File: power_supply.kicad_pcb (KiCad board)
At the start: 2 copper layers, 101.6 x 76.2 mm, 96 parts, among them J1 USB IN, J2 USB OUT, Q1 SI4174DY, Q2 SI4463CDY, Q3 SI4463CDY, U1 LM3914, U10 FDC6392S, U11 MCP6041, U2 TPD2E001, U3 MIC2185, U4 MCP73833, U5 TPD2E001, U6 TPS2511, U7 BATT, U8 LT1389, U9 MAX9938

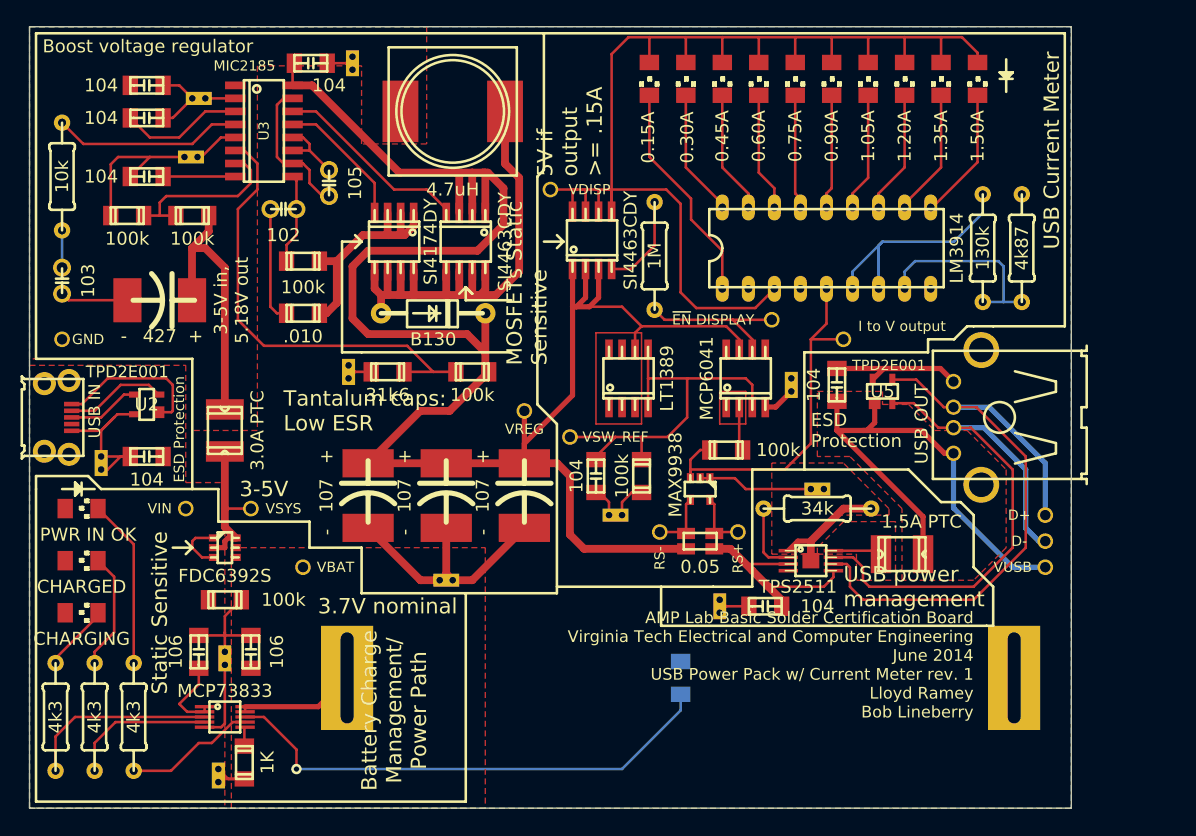
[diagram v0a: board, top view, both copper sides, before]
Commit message: Reshaping board
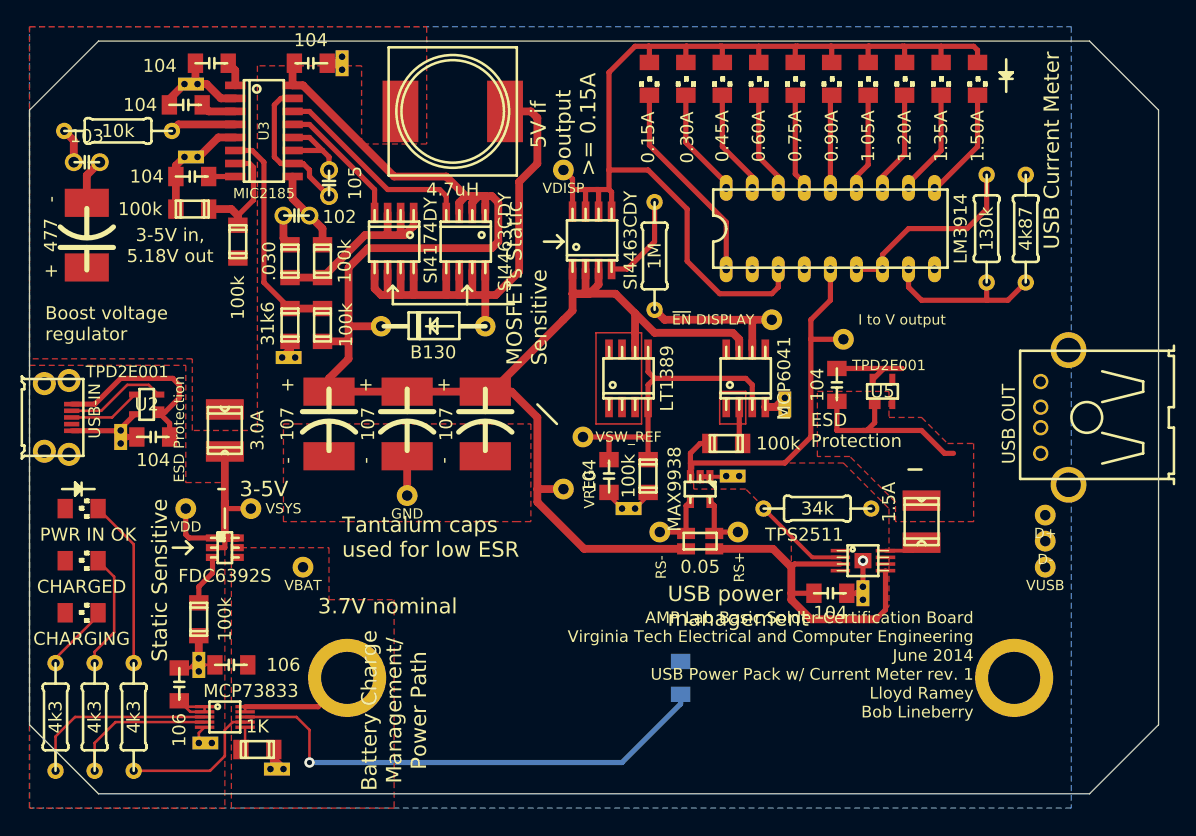
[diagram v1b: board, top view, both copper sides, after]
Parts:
- C1: value 427 -> 477
- D11: value CHARGED -> CHARGED
- F1: value 3.0A PTC -> 3.0A
- F2: value 1.5A PTC -> 1.5A
- J1: value USB IN -> USB-IN
- R10: value .010 -> .030
- RT1: value 10K -> 10K THERMISTOR
- TP1: value VIN -> VDD
- V12: value DV -> DBL_VIA
- moved TP14 36.9 mm to (189.2, 147.3)
- moved V5 28.4 mm to (169.5, 171.4)
- moved R13 15.3 mm to (181.0, 130.7), turned to 270 degrees
- moved V11 14.0 mm to (233.7, 156.8)
- moved C4 11.8 mm to (158.0, 114.8), turned to 0 degrees
- moved R14 10.6 mm to (177.8, 130.7), turned to 90 degrees
- moved C1 9.53 mm to (158.0, 121.9), turned to 90 degrees
- moved TP5 8.52 mm to (204.5, 146.7), turned to 180 degrees
- moved J2 8.51 mm to (262.5, 139.7)
- moved V10 8.35 mm to (221.0, 145.4)
- moved C12 7.96 mm to (196.8, 140.3)
- moved C14 7.96 mm to (189.2, 140.3)
- moved C15 7.96 mm to (181.6, 140.3)
- moved R5 7.04 mm to (161.0, 111.8), turned to 180 degrees
- moved C2 6.71 mm to (170.2, 105.2), turned to 0 degrees
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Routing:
- net /VSS: track 187.9 -> 96.3 mm, vias 0 -> 1
- net /D+: track 64.7 -> 0.00 mm
- net /D-: track 59.9 -> 0.00 mm
- net N-0000068: track 50.7 -> 18.5 mm
- net N-0000049: track 26.7 -> 2.44 mm
- net /VREG: track 219.7 -> 196.4 mm
- net N-0000023: track 44.9 -> 21.8 mm
- net N-0000050: track 18.5 -> 6.44 mm
- net /VDISP: track 117.7 -> 106.5 mm
- net /VOUT: track 21.9 -> 32.7 mm
- net N-0000057: track 12.1 -> 3.49 mm
- net N-0000042: track 39.4 -> 31.8 mm
- net /VDD: track 28.1 -> 34.9 mm
- net N-0000058: track 17.2 -> 11.3 mm
- net N-0000062: track 7.04 -> 2.59 mm
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- removed copper zone on F.Cu, net /VUSB
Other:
- board size 101.6 x 76.2 mm -> 110.1 x 73.4 mm
- board text added: "5V if output >= 0.15A"
- board text added: "Battery Charge Management/Power Path: Controls Li-Ion charge"
- board text added: "Tantalum caps used for low ESR"
- board text added: "external and battery power"
- board text added: "profile (CC @ 1A -> CV @ 4.2V) Automatically switches between"
- board text removed: "5V if output >= .15A"
- board text removed: "Battery Charge Management/Power Path: Controls Li-Ion charge profile (CC @ 1A -> CV @ 4.2V) Automatically switches between external and battery power"
- board text removed: "Tantalum caps: Low ESR"
